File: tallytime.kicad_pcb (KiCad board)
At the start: 4 copper layers, 63.5 x 61 mm, 96 parts, among them IC1 W25Q16JVUXIQ, J1 SH1106 SPI 7PIN, J2 Pico 3PIN SWD, J3 Pico 3PIN UART, J4 BATT, J5 USB_C_Receptacle_USB2.0_16P, J6 TRRS Out, J7 TRRS Out, J8 TALLYLIGHT, Q1 AO3401A, Q2 2N7002, Q3 2N7002, SW1 BOOT, SW2 RESET, SW3 RotaryEncoder_Switch, SW4 SW_SPST, U1 RP2040, U2 TP4056X, U3 AMS1117-3.3, U4 Ai-Thinker-Ra-02, U5 USBLC6-2SC6, U6 LM358, U7 MCP6S91-E_SN, U8 4011, Y1 12MHz +-10ppm 20pF

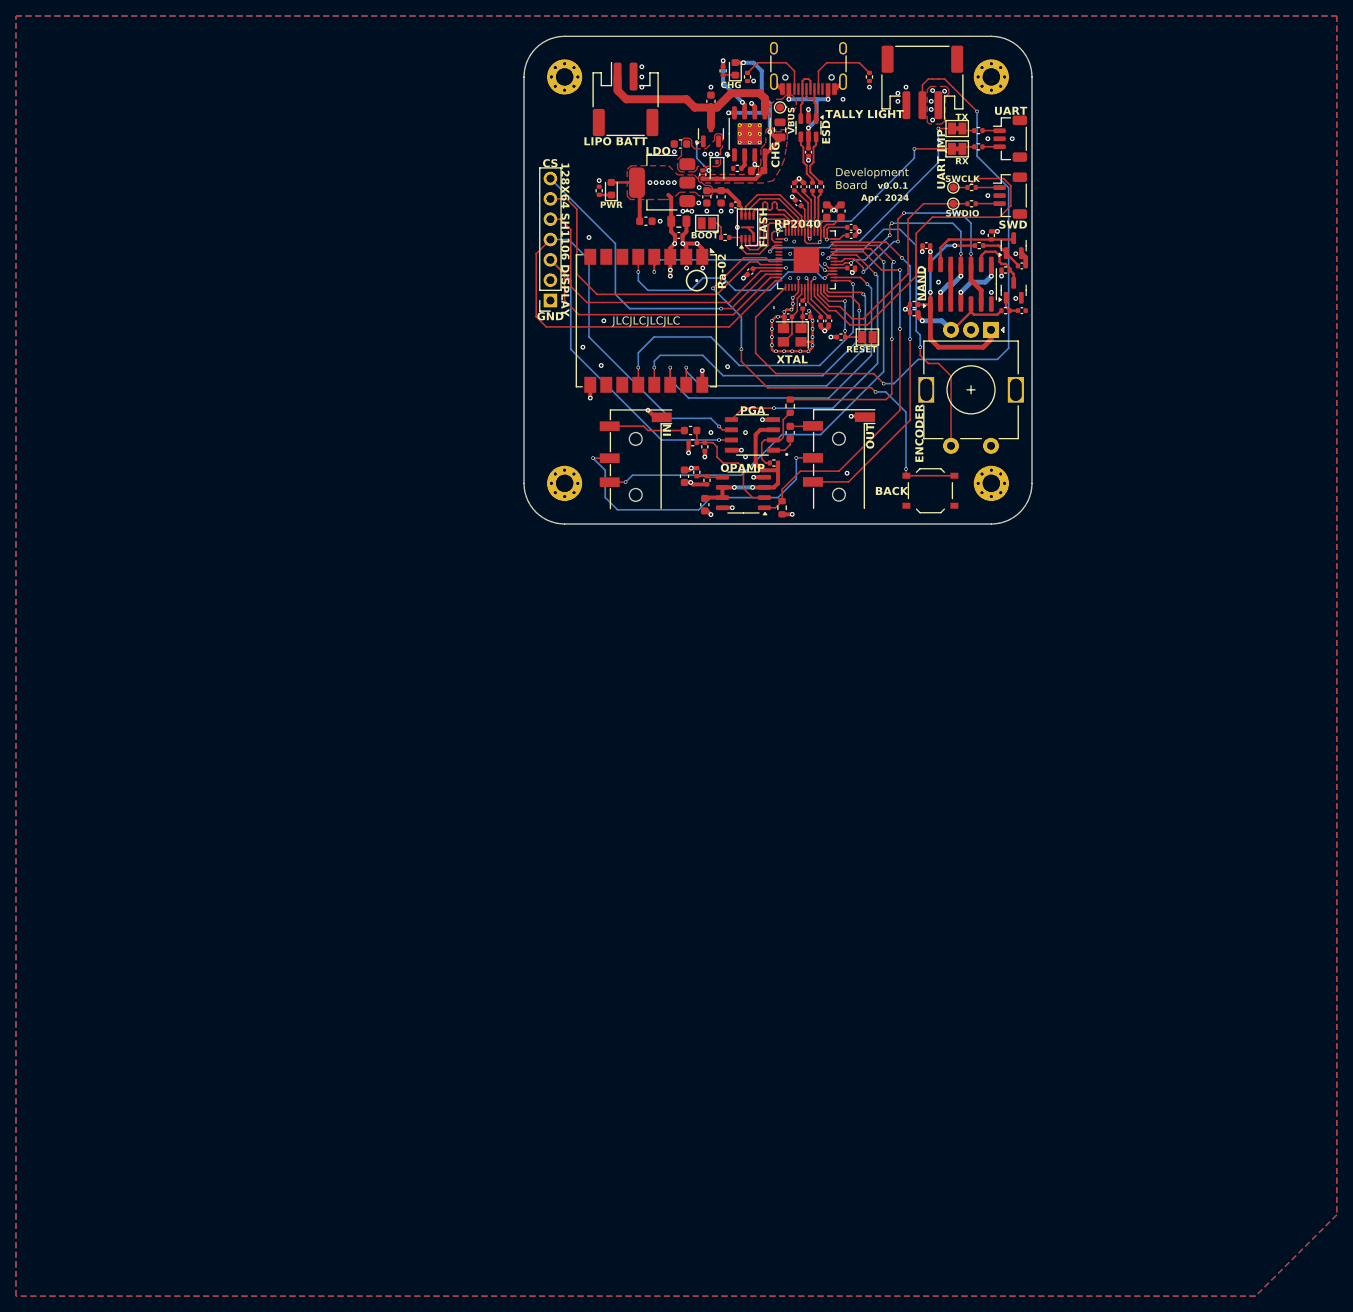
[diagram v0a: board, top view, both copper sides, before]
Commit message: v0.1.0
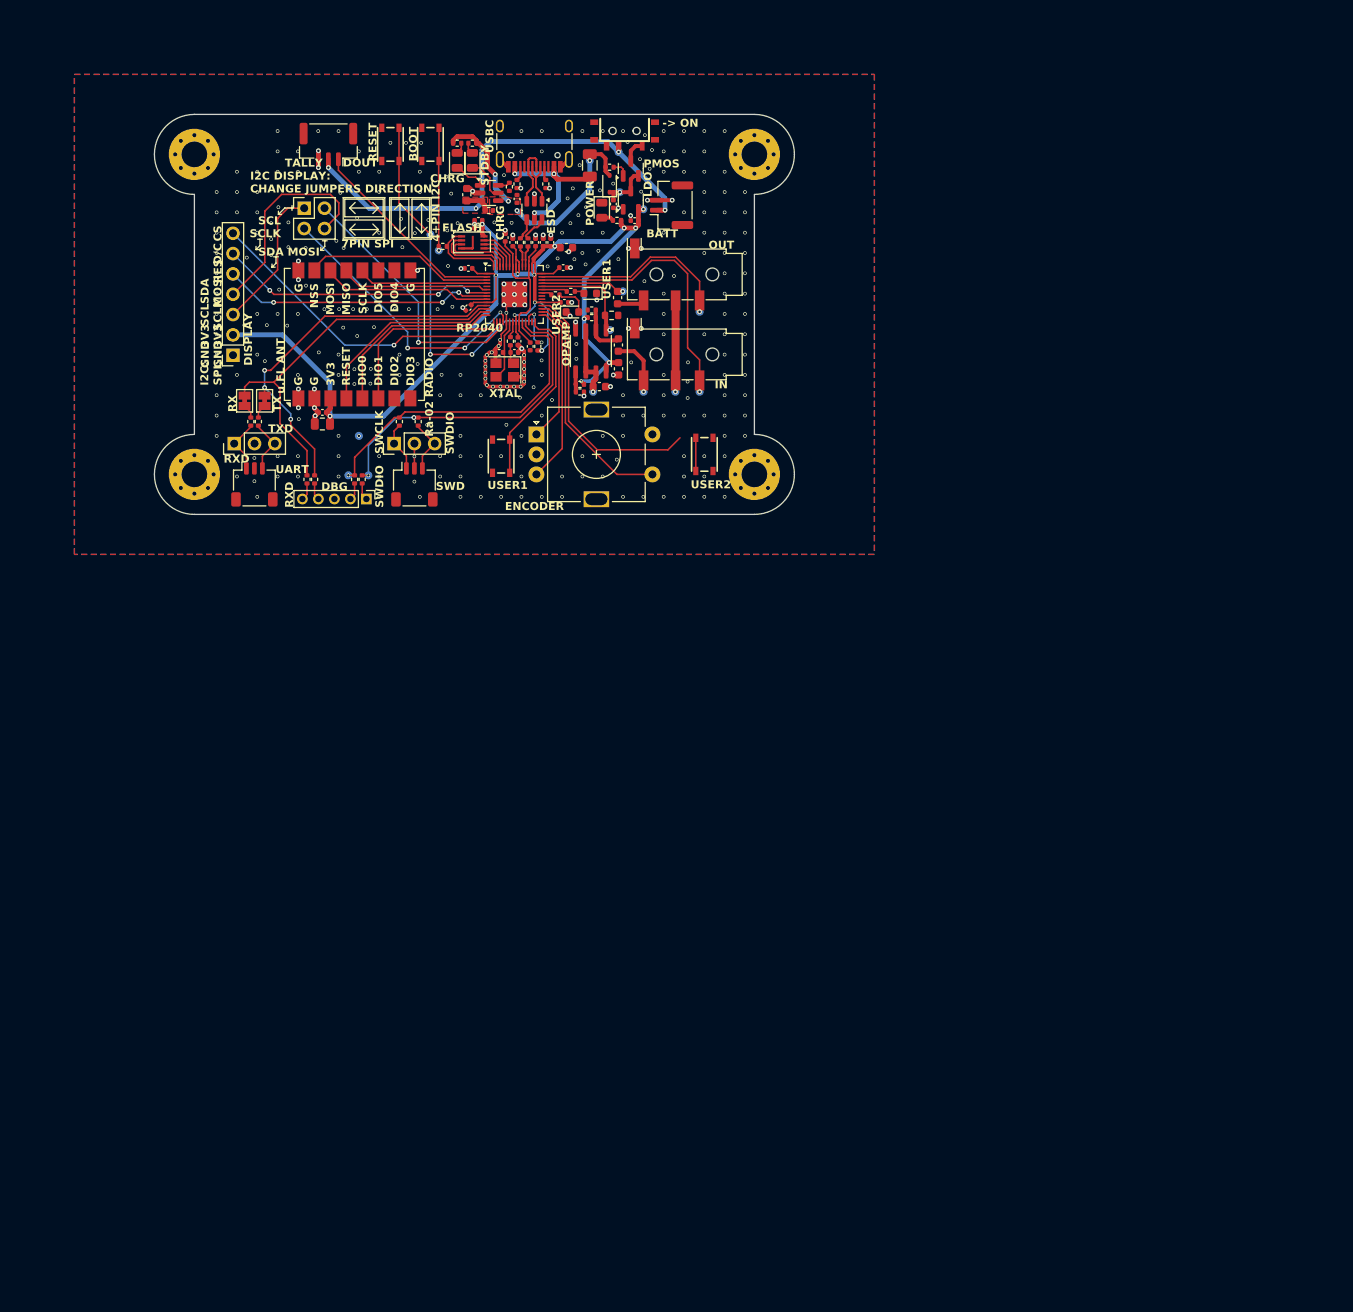
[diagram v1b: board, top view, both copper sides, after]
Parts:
- removed C27, C28, C29, C30: 100n, Capacitor_SMD:C_0402_1005Metric
- removed IC1: W25Q16JVUXIQ, footprints:SON50P300X200X60-9N
- removed Q2, Q3: 2N7002, Package_TO_SOT_SMD:SOT-23
- removed U8: 4011, Package_SO:SOIC-14_3.9x8.7mm_P1.27mm
- added D4: RED, LED_SMD:LED_0805_2012Metric, F.Cu at (85.9, 37.0)
- added D5: GREEN, LED_SMD:LED_0805_2012Metric, F.Cu at (69.8, 30.8)
- added D6: RED, LED_SMD:LED_0805_2012Metric, F.Cu at (67.8, 30.8)
- added J10: OLED DISPLAY, Connector_PinSocket_2.54mm:PinSocket_1x07_P2.54mm_Vertical, F.Cu at (39.8, 55.1)
- added J12: BATT, Connector_JST:JST_GH_SM02B-GHS-TB_1x02-1MP_P1.25mm_Horizontal, F.Cu at (94.7, 36.4)
- added J13: TALLY LIGHT, Connector_JST:JST_GH_SM03B-GHS-TB_1x03-1MP_P1.25mm_Horizontal, F.Cu at (51.8, 28.8)
- added J9: Conn_02x02_Counter_Clockwise, Connector_PinHeader_2.54mm:PinHeader_2x02_P2.54mm_Vertical, F.Cu at (48.7, 36.7)
- added SW5: SKRPACE010, footprints:SKRPACE010, F.Cu at (98.8, 67.5)
- added SW6: SW_SPDT, footprints:SW-SMD_3P-P1.50_L2.7-W6.6, F.Cu at (88.8, 27.5)
- added TP1: VBUS, TestPoint:TestPoint_Pad_D1.0mm, B.Cu at (80.0, 32.4)
- added TP10: MIC, TestPoint:TestPoint_Pad_D1.0mm, B.Cu at (95.1, 59.7)
- added TP11: DET_IN, TestPoint:TestPoint_Pad_D1.0mm, B.Cu at (98.2, 59.7)
- added TP12: DET_OUT, TestPoint:TestPoint_Pad_D1.0mm, B.Cu at (98.2, 49.7)
- added TP13: BATT, TestPoint:TestPoint_Pad_D1.0mm, B.Cu at (88.0, 29.7)
- added TP14: VIN, TestPoint:TestPoint_Pad_D1.0mm, B.Cu at (88.2, 34.7)
- added TP15: 3V3, TestPoint:TestPoint_Pad_D1.0mm, B.Cu at (91.1, 36.9)
- added TP16: 5V, TestPoint:TestPoint_Pad_D1.0mm, B.Cu at (84.4, 30.8)
- added TP17: GND, TestPoint:TestPoint_Pad_D1.0mm, B.Cu at (55.6, 65.2)
- added TP4: BOOT, TestPoint:TestPoint_Pad_D1.0mm, B.Cu at (65.5, 42.0)
- added TP5: RESET, TestPoint:TestPoint_Pad_D1.0mm, B.Cu at (64.5, 40.0)
- added TP6: VREF, TestPoint:TestPoint_Pad_D1.0mm, B.Cu at (84.8, 59.7)
- added TP7: LTC_RX, TestPoint:TestPoint_Pad_D1.0mm, B.Cu at (86.9, 52.0)
- added TP9: LTC_IN, TestPoint:TestPoint_Pad_D1.0mm, B.Cu at (91.2, 59.7)
- C10, C20: value 100n -> 10u; footprint Capacitor_SMD:C_0402_1005Metric -> Capacitor_SMD:C_0603_1608Metric
- C11: value 100n -> 1u
- C12, C23, C24, C26: value 10u -> 1u; footprint Capacitor_SMD:C_0603_1608Metric -> Capacitor_SMD:C_0402_1005Metric
- C13: value 10u -> 2.2u; footprint Capacitor_SMD:C_0603_1608Metric -> Capacitor_SMD:C_0402_1005Metric
- C14: value 10u -> 100n; footprint Capacitor_SMD:C_0603_1608Metric -> Capacitor_SMD:C_0402_1005Metric
- C15, C16: value 10u -> 33p; footprint Capacitor_SMD:C_0603_1608Metric -> Capacitor_SMD:C_0402_1005Metric
- C19: value 2.2u -> 10u
- C21, C22: value 33p -> 10u; footprint Capacitor_SMD:C_0402_1005Metric -> Capacitor_SMD:C_0603_1608Metric
- C3, C5: value 1u -> 100n; footprint Capacitor_SMD:C_0603_1608Metric -> Capacitor_SMD:C_0402_1005Metric
- D1: value Yellow -> USERLED1
- D2: value 1N5819WS -> USERLED2; footprint Diode_SMD:D_SOD-323 -> LED_SMD:LED_0603_1608Metric
- D3: value Red -> 1N5819WS; footprint LED_SMD:LED_0603_1608Metric -> Diode_SMD:D_SOD-323
- F1: value 1A Resettable -> 1.5A; footprint Fuse:Fuse_0805_2012Metric -> Fuse:Fuse_1206_3216Metric
- H1, H2, H3, H4: footprint MountingHole:MountingHole_2.2mm_M2_Pad_Via -> MountingHole:MountingHole_3.2mm_M3_Pad_Via
- J1: value SH1106 SPI 7PIN -> USB_C_Receptacle_USB2.0_16P; footprint Connector_PinSocket_2.54mm:PinSocket_1x07_P2.54mm_Vertical -> Connector_USB:USB_C_Receptacle_HRO_TYPE-C-31-M-12
- J2: value Pico 3PIN SWD -> SWD; footprint Connector_JST:JST_SH_BM03B-SRSS-TB_1x03-1MP_P1.00mm_Vertical -> Connector_PinHeader_2.54mm:PinHeader_1x03_P2.54mm_Vertical
- J3: value Pico 3PIN UART -> SM03B-SRSS-TB; footprint Connector_JST:JST_SH_BM03B-SRSS-TB_1x03-1MP_P1.00mm_Vertical -> Connector_JST:JST_SH_SM03B-SRSS-TB_1x03-1MP_P1.00mm_Horizontal
- J4: value BATT -> 5PIN HOLES; footprint Connector_JST:JST_PH_S2B-PH-SM4-TB_1x02-1MP_P2.00mm_Horizontal -> Connector_PinHeader_2.00mm:PinHeader_1x05_P2.00mm_Vertical
- J5: value USB_C_Receptacle_USB2.0_16P -> UART; footprint Connector_USB:USB_C_Receptacle_HRO_TYPE-C-31-M-12 -> Connector_PinHeader_2.54mm:PinHeader_1x03_P2.54mm_Vertical
- J6: value TRRS Out -> SM03B-SRSS-TB; footprint Connector_Audio:Jack_3.5mm_KoreanHropartsElec_PJ-320D-4A_Horizontal -> Connector_JST:JST_SH_SM03B-SRSS-TB_1x03-1MP_P1.00mm_Horizontal
- J8: value TALLYLIGHT -> TRRS Out; footprint Connector_JST:JST_PH_S3B-PH-SM4-TB_1x03-1MP_P2.00mm_Horizontal -> Connector_Audio:Jack_3.5mm_KoreanHropartsElec_PJ-320D-4A_Horizontal
- R10, R9: value 1k -> 100
- R11, R12: value 5k1 -> 100
- R13, R14: value 22 -> 100
- R15: value 10k -> 100
- R16, R17, R23, R24, R25, R26: value 10k -> 5k1
- R19, R20: value 150k -> 10k; footprint Resistor_SMD:R_0603_1608Metric -> Resistor_SMD:R_0402_1005Metric
- R2: value 1k1 -> 1k
- R21: value 10k -> 150k; footprint Resistor_SMD:R_0402_1005Metric -> Resistor_SMD:R_0603_1608Metric
- R22: value 1k -> 10k
- R28: value 5k1 -> 2k
- R4: value 1k -> 5k1
- R5: value 100 -> 5k1
- R6, R7: value 100 -> 22
- SW1: value BOOT -> SKRPACE010; footprint Jumper:SolderJumper-2_P1.3mm_Open_Pad1.0x1.5mm -> footprints:SKRPACE010
- SW2: value RESET -> SKRPACE010; footprint Jumper:SolderJumper-2_P1.3mm_Open_Pad1.0x1.5mm -> footprints:SKRPACE010
- SW3: value RotaryEncoder_Switch -> EC11
- SW4: value SW_SPST -> SKRPACE010; footprint Button_Switch_SMD:SW_Push_1P1T_XKB_TS-1187A -> footprints:SKRPACE010
- TP2, TP3: moved to B.Cu
- TP8: value VBUS -> LTC_TX; moved to B.Cu
- U1: value RP2040 -> W25Q16JVUXIQ; footprint Package_DFN_QFN:QFN-56-1EP_7x7mm_P0.4mm_EP3.2x3.2mm -> footprints:SON50P300X200X60-9N
- U2: value TP4056X -> RP2040; footprint Package_SO:Infineon_PG-DSO-8-27_3.9x4.9mm_EP2.65x3mm_ThermalVias -> Package_DFN_QFN:QFN-56-1EP_7x7mm_P0.4mm_EP3.2x3.2mm
- U3: value AMS1117-3.3 -> USBLC6-2SC6; footprint Package_TO_SOT_SMD:SOT-223-3_TabPin2 -> Package_TO_SOT_SMD:SOT-23-6
- U5: value USBLC6-2SC6 -> LM358; footprint Package_TO_SOT_SMD:SOT-23-6 -> Package_SO:SOP-8_3.9x4.9mm_P1.27mm
- U6: value LM358 -> XC6206P332MR; footprint Package_SO:SOP-8_3.9x4.9mm_P1.27mm -> Package_TO_SOT_SMD:SOT-23-3
- U7: value MCP6S91-E_SN -> TP4057; footprint footprints:SOIC127P600X175-8N -> Package_TO_SOT_SMD:SOT-23-6
- moved H3 99.6 mm to (35.0, 70.0)
- moved JP1 95.4 mm to (41.3, 60.8), turned to -90 degrees
- moved JP2 92.1 mm to (43.8, 60.8), turned to -90 degrees
- moved R8 87.5 mm to (56.0, 70.6), turned to 90 degrees
- moved J5 86.6 mm to (40.0, 66.2), turned to 90 degrees
- moved J3 86.1 mm to (62.5, 71.2), turned to 0 degrees
- moved TP2 83.7 mm to (54.2, 70.1), turned to 180 degrees
- moved J2 83.0 mm to (60.0, 66.2), turned to 90 degrees
- moved TP3 80.6 mm to (56.8, 70.1), turned to 180 degrees
- moved SW4 80.2 mm to (59.5, 28.8), turned to -90 degrees
- moved R14 76.1 mm to (42.0, 63.4), turned to 90 degrees
- moved R13 73.9 mm to (49.1, 70.6), turned to 90 degrees
- moved R12 73.9 mm to (50.0, 70.6), turned to 90 degrees
- moved J6 73.2 mm to (42.5, 71.2), turned to 0 degrees
- moved R11 71.0 mm to (63.0, 63.4), turned to 90 degrees
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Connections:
- C11 pad 1: +3V3 -> +1V1
- C13 pad 1: +5V -> +3V3
- C14 pad 1: +BATT -> +3V3
- C15 pad 1: +VIN -> GND
- C15 pad 2: GND -> /MCU/XIN
- C16 pad 1: +3V3 -> GND
- C16 pad 2: GND -> /MCU/XTAL_XOUT
- C20 pad 1: +3V3 -> /Timecode/VREF
- C21 pad 1: GND -> /Timecode/LTC_IN
- C21 pad 2: /MCU/Crystal/XTAL_IN -> /Timecode/OPAMP_A_N
- C22 pad 1: GND -> /MCU/GPIO27_ADC1
- C22 pad 2: /MCU/Crystal/XTAL_O -> /Timecode/LTC_OUT
- C23 pad 1: /TimecodeIO/LTC_OUT_DC -> +VIN
- C23 pad 2: /TimecodeIO/LTC_OUT -> GND
- C24 pad 1: /TimecodeIO/LTC_IN -> +3V3
- C24 pad 2: /TimecodeIO/OPAMP_A_N -> GND
- C25 pad 1: +3V3 -> +BATT
- C26 pad 1: /TimecodeIO/VREF -> +5V
- C3 pad 1: +1V1 -> +3V3
- D1 pad 1: /Power/CHRG_STAT_1 -> GND
- D1 pad 2: +5V -> /Debug/USERLED1_K
- D2 pad 1: +VIN -> GND
- D2 pad 2: +5V -> /Debug/USERLED2_K
- D3 pad 1: Net-(D3-K) -> +VIN
- D3 pad 2: +3V3 -> +5V
- J2 pad 1: Net-(J2-Pin_1) -> /Debug/3PIN_SWD_SWCLK
- J2 pad 3: Net-(J2-Pin_3) -> /Debug/3PIN_SWD_SWDIO
- J3 pad 1: Net-(J3-Pin_1) -> /Debug/3PIN_SWD_SWCLK
- J3 pad 3: Net-(J3-Pin_3) -> /Debug/3PIN_SWD_SWDIO
- J3 pad MP: GND -> unconnected-(J3-MountPin-PadMP)
- J4 pad 1: +BATT -> /Debug/5PIN_SWD_SWDIO
- J4 pad 2: GND -> /Debug/5PIN_SWD_SWCLK
- J7 pad R1: /TimecodeIO/MIC_PASSTHROUGH -> /Timecode/MIC_PASSTHROUGH
- J7 pad R2: /MCU/DET_IN -> /MCU/GPIO28_ADC2
- J7 pad T: /TimecodeIO/LTC_IN -> /Timecode/LTC_IN
- JP1 pad 1: /MCU/UART0_RX -> /Debug/UART_RX
- JP1 pad 2: /Interfaces/UART_RX -> /Debug/JMP_UART_RX
- JP2 pad 1: /MCU/UART0_TX -> /Debug/UART_TX
- JP2 pad 2: /Interfaces/UART_TX -> /Debug/JMP_UART_TX
- Q1 pad 3: +BATT -> /Power/BATT_SW
- R1 pad 2: /Interfaces/~{RESET} -> /Debug/~{RESET}
- R10 pad 1: /MCU/Crystal/XTAL_O -> /Debug/5PIN_SWD_SWCLK
- R10 pad 2: /MCU/Crystal/XOUT -> /Debug/SWCLK
- R11 pad 1: Net-(J5-CC1) -> /Debug/3PIN_SWD_SWDIO
- R11 pad 2: GND -> /Debug/SWDIO
- R12 pad 1: Net-(J5-CC2) -> /Debug/5PIN_UART_TX
- R12 pad 2: GND -> /Debug/UART_TX
- R13 pad 1: /MCU/USB/USBESD- -> /Debug/5PIN_UART_RX
- R13 pad 2: /MCU/USB/USB_D- -> /Debug/UART_RX
- R14 pad 1: /MCU/USB/USBESD+ -> /Debug/3PIN_UART_RX
- R14 pad 2: /MCU/USB/USB_D+ -> /Debug/JMP_UART_RX
- R15 pad 1: +3V3 -> /Debug/3PIN_UART_TX
- R15 pad 2: /TimecodeIO/OPAMP_A_N -> /Debug/JMP_UART_TX
- R16 pad 1: /TimecodeIO/OPAMP_A_N -> /Debug/USERLED1
- R16 pad 2: GND -> /Debug/USERLED1_K
- R17 pad 1: +3V3 -> /Debug/USERLED2
- R17 pad 2: /TimecodeIO/OPAMP_B_P -> /Debug/USERLED2_K
- R18 pad 1: /TimecodeIO/OPAMP_B_P -> +3V3
- R18 pad 2: GND -> /Timecode/OPAMP_B_P
- R19 pad 1: /MCU/LTC_RX -> /Timecode/OPAMP_B_P
- R2 pad 1: /Power/CHRG_ISET -> /Debug/~{BOOT}
- R2 pad 2: GND -> /MCU/QSPI_SS
- R20 pad 1: /MCU/LTC_TX -> +3V3
- R20 pad 2: /TimecodeIO/LTC_CH0 -> /Timecode/OPAMP_A_N
- R21 pad 1: /TimecodeIO/LTC_CH0 -> /MCU/GPIO26_ADC0
- R21 pad 2: /TimecodeIO/VREF -> GND
- R22 pad 1: Net-(D3-K) -> /Timecode/OPAMP_A_N
- R23 pad 1: +3V3 -> +5V
- R23 pad 2: Net-(R23-Pad2) -> /Power/MOS_BIAS
- R24 pad 2: Net-(Q2-D) -> /Power/POWER_LED_K
- R25 pad 1: +3V3 -> +5V
- R25 pad 2: Net-(R25-Pad2) -> Net-(D5-A)
- R26 pad 1: +3V3 -> +5V
- R27 pad 1: Net-(R25-Pad2) -> +5V
- R27 pad 2: Net-(Q3-G) -> +BATT
- R28 pad 1: Net-(R23-Pad2) -> Net-(U7-PROG)
- R28 pad 2: Net-(Q2-G) -> GND
- R3 pad 1: /Power/CHRG_STAT_1 -> /MCU/XTAL_XOUT
- R3 pad 2: Net-(U2-~{CHRG}) -> /MCU/XOUT
- R4 pad 1: +5V -> /USB/USB_CC1
- R4 pad 2: /Power/MOS_BIAS -> GND
- R5 pad 1: Net-(J2-Pin_1) -> /USB/USB_CC2
- R5 pad 2: /Interfaces/SWCLK -> GND
- R6 pad 1: Net-(J2-Pin_3) -> /USB/USBESD-
- R6 pad 2: /Interfaces/SWDIO -> /MCU/USB_D-
- R7 pad 1: Net-(J3-Pin_1) -> /USB/USBESD+
- R7 pad 2: /Interfaces/UART_RX -> /MCU/USB_D+
- R8 pad 1: Net-(J3-Pin_3) -> /Debug/5PIN_SWD_SWDIO
- R8 pad 2: /Interfaces/UART_TX -> /Debug/SWDIO
- R9 pad 1: /Interfaces/~{BOOT} -> /Debug/3PIN_SWD_SWCLK
- R9 pad 2: /MCU/Flash/QSPI_SS -> /Debug/SWCLK
- SW1 pad 1: /Interfaces/~{BOOT} -> /Debug/~{BOOT}
- SW2 pad 1: /Interfaces/~{RESET} -> /Debug/USERSW1
- SW3 pad A: Net-(R23-Pad2) -> /Debug/ENCODER_A
- SW3 pad B: Net-(R25-Pad2) -> /Debug/ENCODER_B
- SW3 pad MP: (no net) -> unconnected-(SW3-PadMP)_0
- SW3 pad S1: /Interfaces/ENC_SW -> /Debug/ENCODER_SW
- SW4 pad 1: GND -> /Debug/~{RESET}
- SW4 pad 2: /Interfaces/SW_BACK -> GND
- TP2 pad 1: /Interfaces/SWCLK -> /Debug/SWCLK
- TP3 pad 1: /Interfaces/SWDIO -> /Debug/SWDIO
- TP8 pad 1: VBUS -> /MCU/GPIO27_ADC1
- U1 pad 1: +3V3 -> /MCU/QSPI_SS
- U1 pad 2: /MCU/UART0_TX -> /MCU/QSPI_SD1
- U1 pad 3: /MCU/UART0_RX -> /MCU/QSPI_SD2
- U1 pad 4: unconnected-(U1-GPIO2-Pad4) -> GND
- U1 pad 5: unconnected-(U1-GPIO3-Pad5) -> /MCU/QSPI_SD0
- U1 pad 6: unconnected-(U1-GPIO4-Pad6) -> /MCU/QSPI_SCLK
- U1 pad 7: unconnected-(U1-GPIO5-Pad7) -> /MCU/QSPI_SD3
- U1 pad 8: /Interfaces/SW_BACK -> +3V3
- U1 pad 9: /Display/DC -> GND
- U2 pad 1: GND -> +3V3
- U2 pad 2: /Power/CHRG_ISET -> /Debug/TALLY
- U2 pad 3: GND -> /MCU/GPIO1
- U2 pad 4: +5V -> /MCU/GPIO2
- U2 pad 5: +BATT -> /MCU/GPIO3
- U2 pad 6: GND -> /MCU/GPIO4
- U2 pad 7: Net-(U2-~{CHRG}) -> /Display/D/C
- U2 pad 8: +5V -> /Display/RES
- U2 pad 9: GND -> /MCU/GPIO7
- U3 pad 1: GND -> /USB/USBD-
- U3 pad 2: +3V3 -> GND
- U3 pad 3: +VIN -> /USB/USBD+
- U4 pad 10: unconnected-(U4-DIO4-Pad10) -> /Radio/DIO4
- U4 pad 11: unconnected-(U4-DIO5-Pad11) -> /Radio/DIO5
- U4 pad 12: /MCU/SPI0.SCK -> /MCU/GPIO2
- U4 pad 13: /MCU/SPI0.MISO -> /MCU/GPIO4
- U4 pad 14: /MCU/SPI0.MOSI -> /MCU/GPIO7
- U4 pad 15: /MCU/SPI0_CS1 -> /MCU/GPIO1
- U4 pad 4: /MCU/GPIO21 -> /MCU/GPIO10
- U4 pad 5: /MCU/GPIO20 -> /MCU/GPIO11
- U4 pad 6: unconnected-(U4-DIO1-Pad6) -> /MCU/GPIO12
- U4 pad 7: unconnected-(U4-DIO2-Pad7) -> /Radio/DIO2
- U4 pad 8: unconnected-(U4-DIO3-Pad8) -> /Radio/DIO3
- U5 pad 1: /MCU/USB/USBD- -> /MCU/GPIO26_ADC0
- U5 pad 2: GND -> /Timecode/OPAMP_A_N
- U5 pad 3: /MCU/USB/USBD+ -> /Timecode/VREF
- U5 pad 4: /MCU/USB/USBESD+ -> GND
- U5 pad 5: VBUS -> /Timecode/OPAMP_B_P
- U5 pad 6: /MCU/USB/USBESD- -> /Timecode/VREF
- U6 pad 1: /MCU/LTC_RX -> GND
- U6 pad 2: /TimecodeIO/OPAMP_A_N -> +3V3
- U6 pad 3: /TimecodeIO/VREF -> +VIN
- U7 pad 1: /TimecodeIO/LTC_OUT_DC -> Net-(D6-K)
- U7 pad 2: /TimecodeIO/LTC_CH0 -> GND
- U7 pad 3: /TimecodeIO/VREF -> +BATT
- U7 pad 4: GND -> +5V
- U7 pad 5: /MCU/SPI1_CS2 -> Net-(D5-K)
- U7 pad 6: /MCU/SPI1.MOSI -> Net-(U7-PROG)
- Y1 pad 1: /MCU/Crystal/XTAL_O -> /MCU/XTAL_XOUT
- Y1 pad 3: /MCU/Crystal/XTAL_IN -> /MCU/XIN
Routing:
- net +3V3: track 75.7 -> 163.8 mm, vias 24 -> 15
- net /Interfaces/TALLY_OUT: track 87.4 -> 0.00 mm, vias 2 -> 0
- net /MCU/SPI1.MOSI: track 81.8 -> 0.00 mm, vias 1 -> 0
- net /MCU/SPI1.SCK: track 72.3 -> 0.00 mm, vias 1 -> 0
- net /MCU/DET_IN: track 60.6 -> 0.00 mm, vias 2 -> 0
- net /Interfaces/SW_BACK: track 57.8 -> 0.00 mm, vias 4 -> 0
- net /Debug/~{RESET}: track 0.00 -> 50.8 mm, vias 0 -> 5
- net /MCU/LTC_RX: track 49.6 -> 0.00 mm, vias 2 -> 0
- net /Debug/UART_RX: track 0.00 -> 48.8 mm
- net /Debug/UART_TX: track 0.00 -> 47.8 mm, vias 0 -> 3
- net /Interfaces/SWCLK: track 47.0 -> 0.00 mm
- net /MCU/SPI0.MOSI: track 45.6 -> 0.00 mm, vias 2 -> 0
- net /MCU/DET_OUT: track 45.4 -> 0.00 mm, vias 2 -> 0
- net /MCU/SPI0.SCK: track 43.4 -> 0.00 mm, vias 2 -> 0
- net /MCU/SPI0.MISO: track 41.8 -> 0.00 mm, vias 2 -> 0
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- added copper zone on F.Cu, net +BATT
- added copper zone on In2.Cu, net GND
- removed copper zone on F.Cu, net +3V3
- removed copper zone on In2.Cu, net +3V3
- removed copper zone on F.Cu, net +VIN
- removed copper zone on In2.Cu, net +VIN
- removed copper zone on F.Cu, net VBUS
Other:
- board size 63.5 x 61 mm -> 80 x 50 mm
- board text added: "-> ON"
- board text added: "3V3"
- board text added: "3V3 3V3"
- board text added: "4+PIN I2C"
- board text added: "5V"
- board text added: "7PIN SPI"
- board text added: "@plushugh"
- board text added: "BATT"
- board text added: "CHRG"
- board text added: "D/C"
- board text added: "DBG"
- board text added: "DET_IN"
- board text added: "DIO0"
- board text added: "DIO1"
- board text added: "DIO2"
- board text added: "DIO3"
- board text added: "DIO4"
- board text added: "DIO5"
- board text added: "DISPLAY"
- board text added: "DOUT"
- board text added: "G"
- board text added: "GND GND"
- board text added: "I2C DISPLAY: CHANGE JUMPERS DIRECTION"
- board text added: "I2C:"
- board text added: "LTC_IN"
- board text added: "LTC_RX"
- board text added: "LTC_TX"
- board text added: "MIC"
- board text added: "MISO"
- board text added: "MOSI"
- board text added: "NSS"
- board text added: "PMOS"
- board text added: "POWER"
- board text added: "RES"
- board text added: "RXD"
- board text added: "Ra-02 RADIO"
- board text added: "SCL SCLK"
- board text added: "SCLK"
- board text added: "SDA MOSI"
- board text added: "SPI:"
- board text added: "STDBY"
- board text added: "TALLY"
- board text added: "TXD"
- board text added: "USBC"
- board text added: "USER1"
- board text added: "USER2"
- board text added: "VIN"
- board text added: "VREF"
- board text added: "u.FL ANT"
- board text added: "v0.1.0"
- board text added: "© MicroHenry 2024 June"
- board text removed: "128X64 SH1106 DISPLAY"
- board text removed: "Apr. 2024"
- board text removed: "BACK"
- board text removed: "CHG"
- board text removed: "GND"
- board text removed: "JLCJLCJLCJLC"
- board text removed: "LIPO BATT"
- board text removed: "NAND"
- board text removed: "PGA"
- board text removed: "PWR"
- board text removed: "Ra-02"
- board text removed: "TALLY LIGHT"
- board text removed: "UART JMP"
- board text removed: "v0.0.1"
